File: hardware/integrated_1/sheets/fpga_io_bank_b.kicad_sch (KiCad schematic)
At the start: 22 parts, among them U1 XC6SLX9-TQG144, U2 IS25LP128F-JBLE-TR

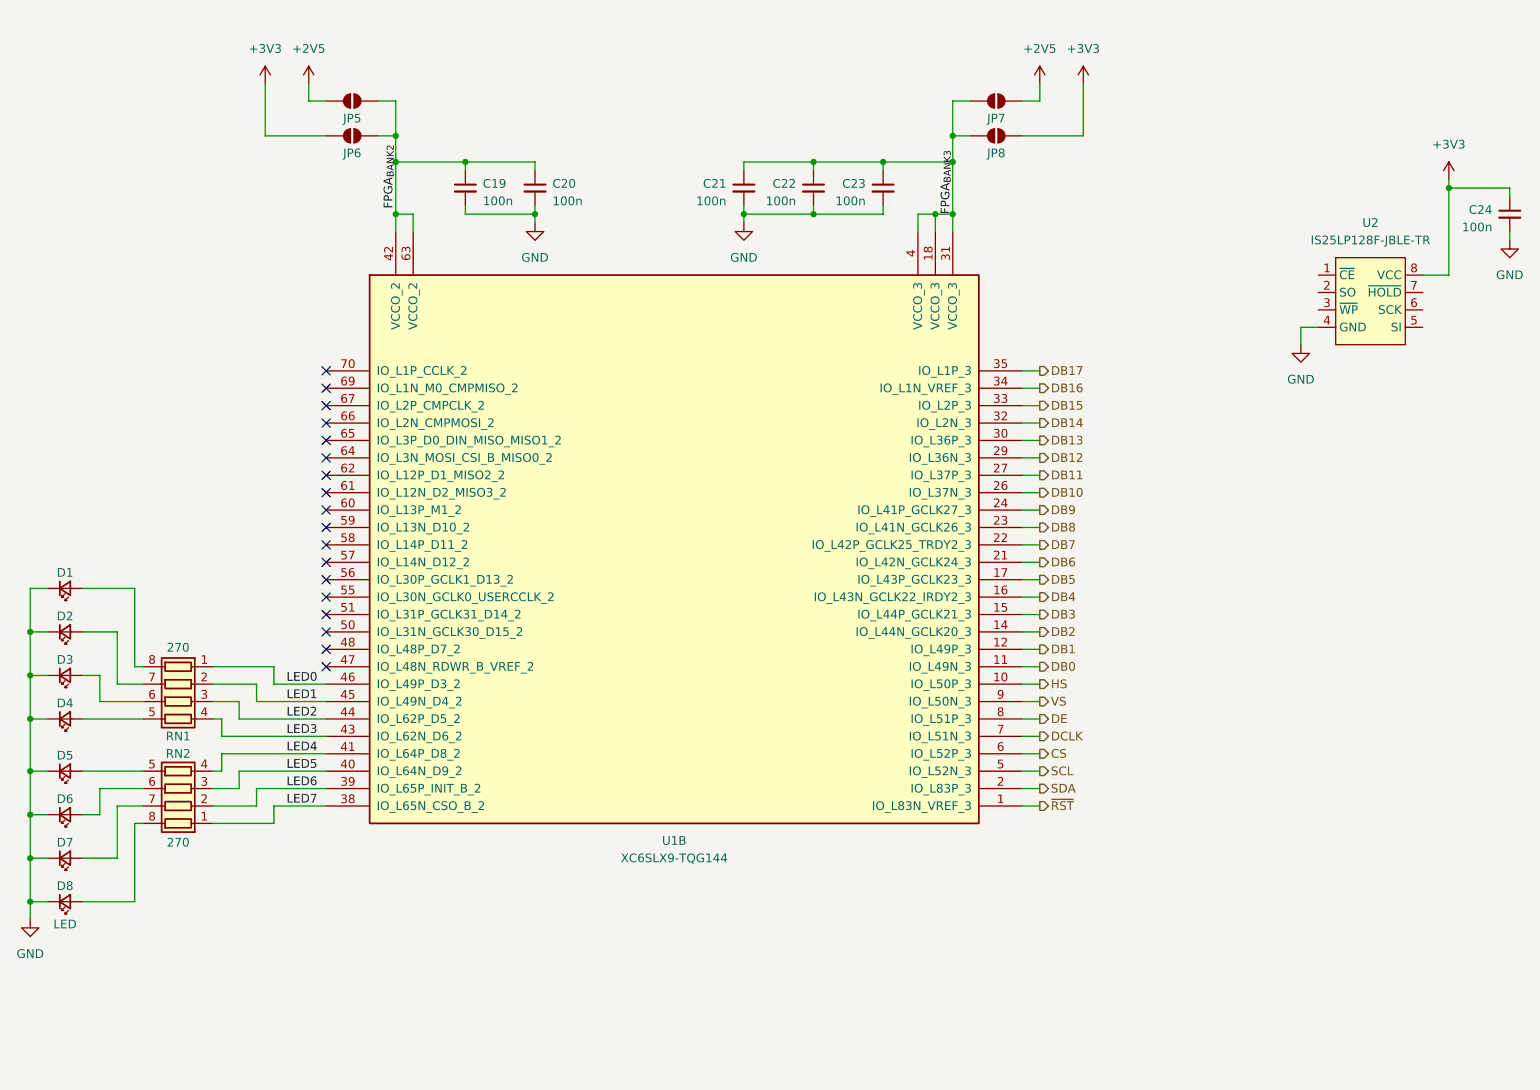
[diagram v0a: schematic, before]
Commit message: finalizing the schematic and layout
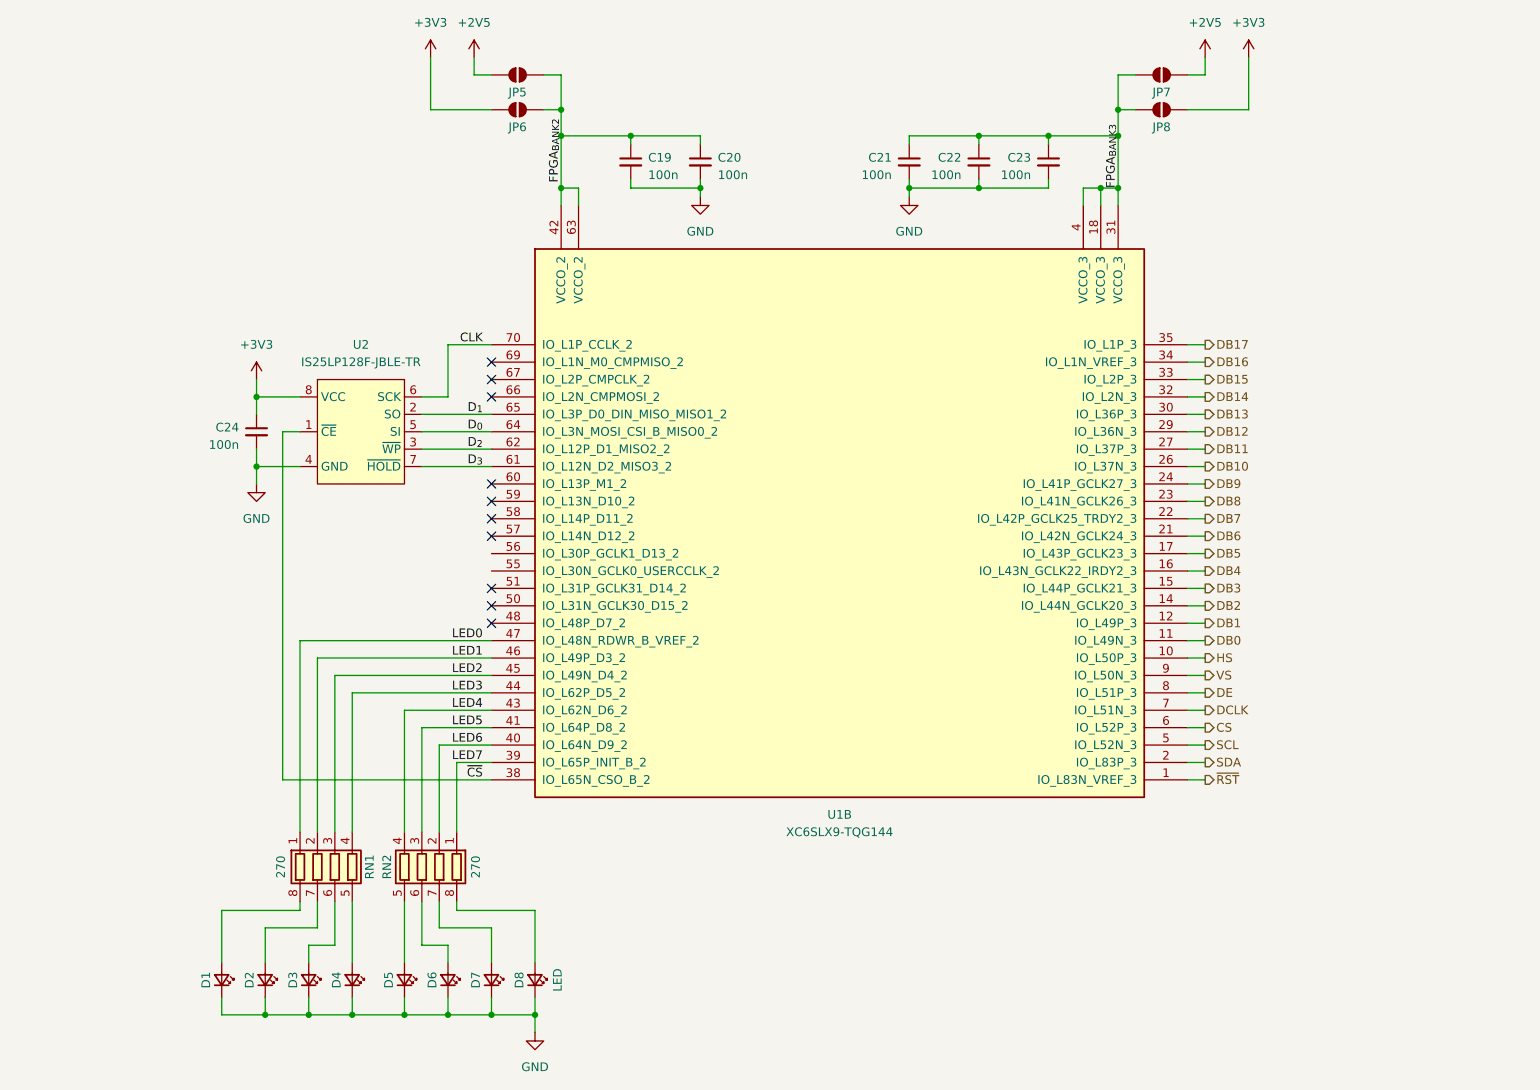
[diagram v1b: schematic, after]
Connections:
- net LED0: now also U1.47 (IO_L48N_RDWR_B_VREF_2); no longer U1.46 (IO_L49P_D3_2)
- net LED1: now also U1.46 (IO_L49P_D3_2); no longer U1.45 (IO_L49N_D4_2)
- net LED2: now also U1.45 (IO_L49N_D4_2); no longer U1.44 (IO_L62P_D5_2)
- net LED3: now also U1.44 (IO_L62P_D5_2); no longer U1.43 (IO_L62N_D6_2)
- net LED4: now also U1.43 (IO_L62N_D6_2); no longer U1.41 (IO_L64P_D8_2)
- net LED5: now also U1.41 (IO_L64P_D8_2); no longer U1.40 (IO_L64N_D9_2)
- net LED6: now also U1.40 (IO_L64N_D9_2); no longer U1.39 (IO_L65P_INIT_B_2)
- net LED7: now also U1.39 (IO_L65P_INIT_B_2); no longer U1.38 (IO_L65N_CSO_B_2)
- net ~{CS}: now reaches U2.1 (~{CE})
- net ~{CS}: now also U1.38 (IO_L65N_CSO_B_2)
- net D_{1}: now reaches U2.2 (SO)
- net D_{1}: now also U1.65 (IO_L3P_D0_DIN_MISO_MISO1_2)
- net D_{2}: now reaches U2.3 (~{WP})
- net D_{2}: now also U1.62 (IO_L12P_D1_MISO2_2)
- net D_{0}: now reaches U2.5 (SI)
- net D_{0}: now also U1.64 (IO_L3N_MOSI_CSI_B_MISO0_2)
- net CLK: now reaches U2.6 (SCK)
- net CLK: now also U1.70 (IO_L1P_CCLK_2)
- net D_{3}: now reaches U2.7 (~{HOLD})
- net D_{3}: now also U1.61 (IO_L12N_D2_MISO3_2)
- no-connect marks 18 -> 10
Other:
- moved on the sheet: C19, C20, C21, C22, C23, C24, D1, D2, D3, D4, D5, D6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
